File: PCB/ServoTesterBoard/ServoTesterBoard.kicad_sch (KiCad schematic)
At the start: 23 parts, among them J1 Barrel Jack, J2 2.54mm 1x2 Header, J3 2.54mm 1x3 Header, Q1 BC547, SW1 Slide Switch, SW2 Push Button, SW3 Push Button, U1 LM555xM, U2 L7805

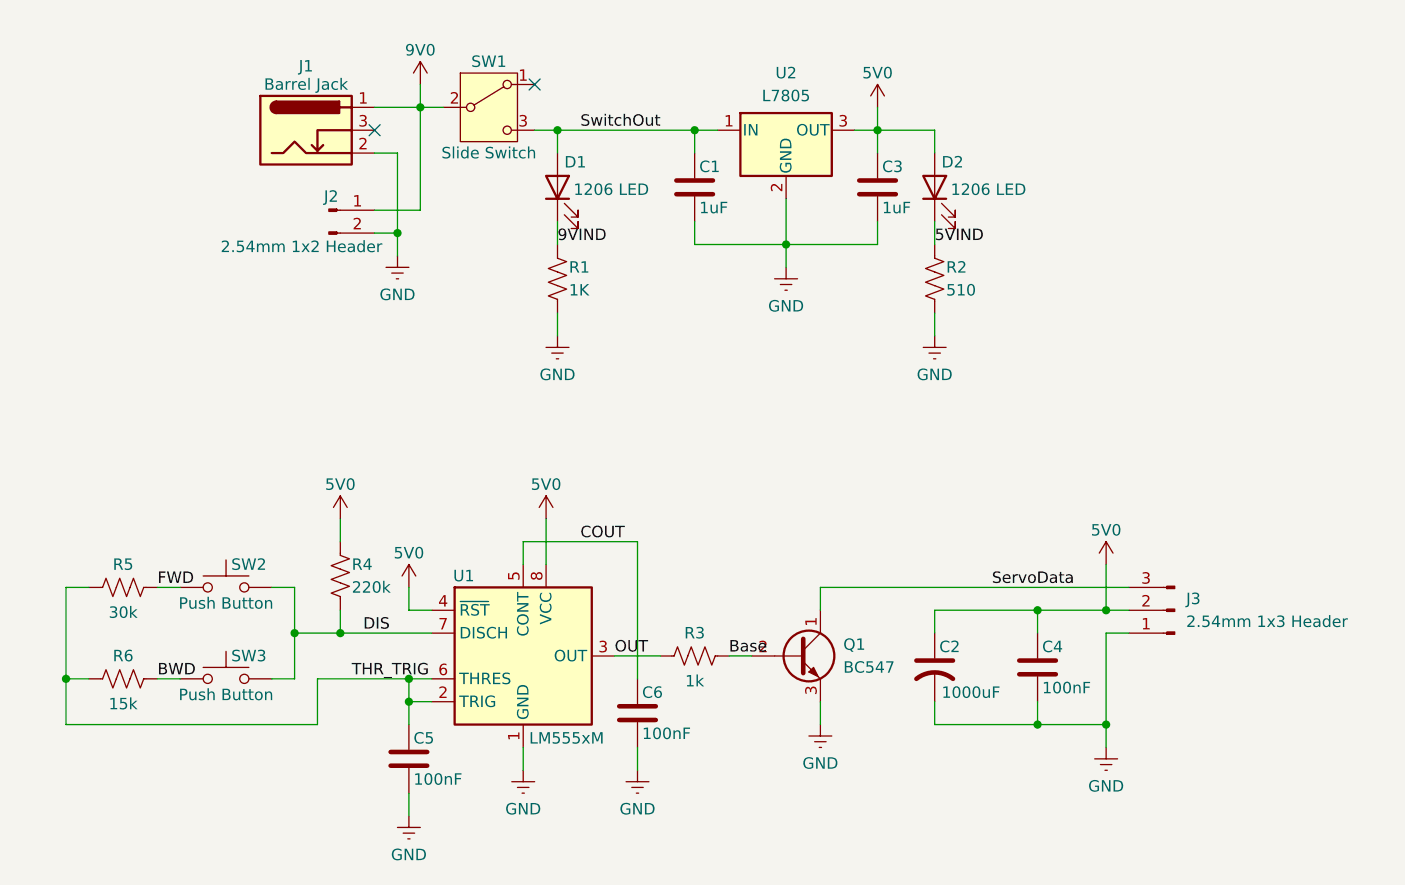
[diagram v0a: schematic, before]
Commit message: Finished
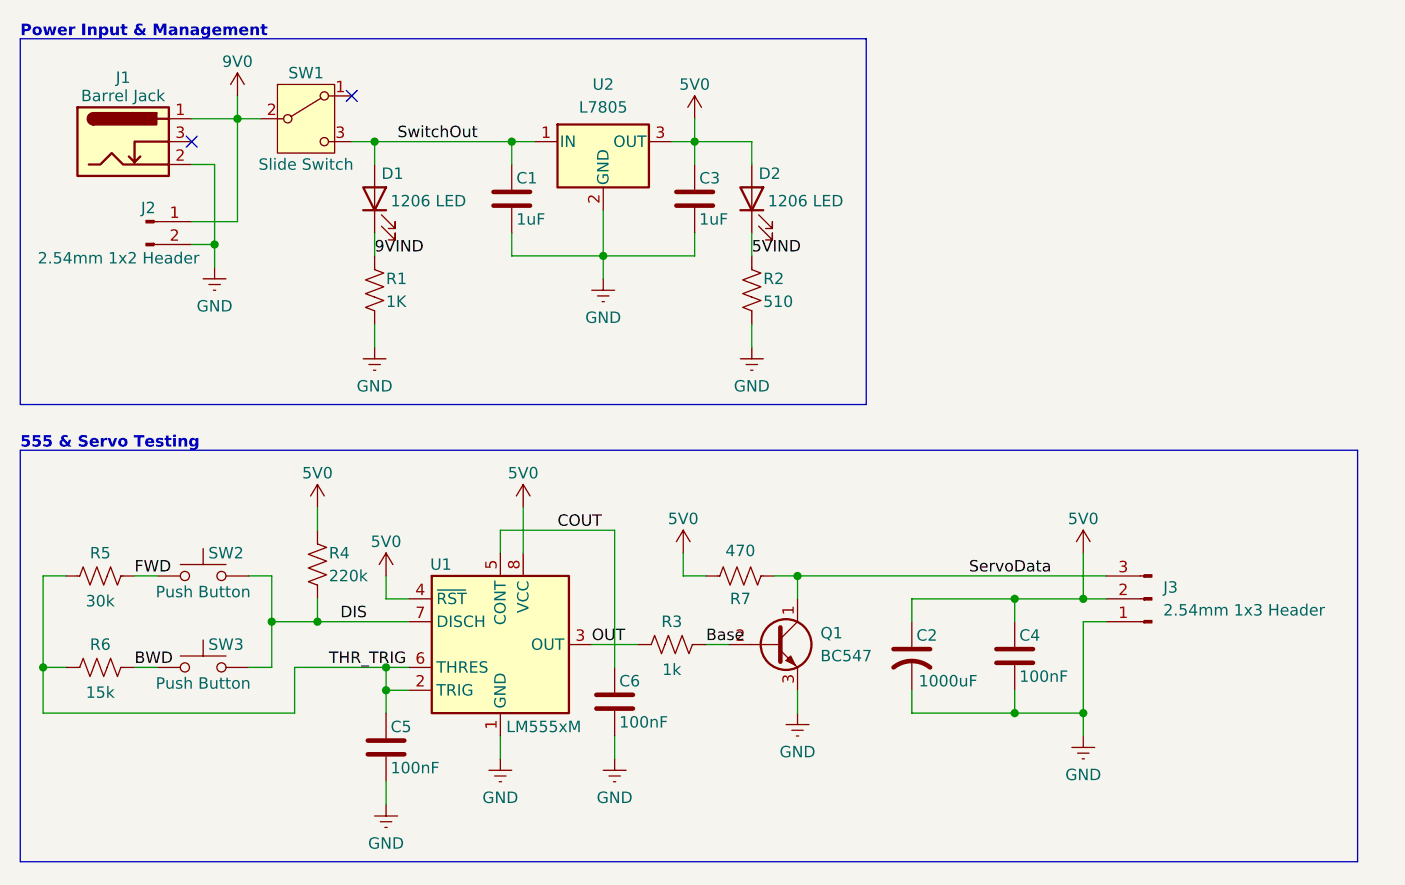
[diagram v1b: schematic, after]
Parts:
- added R7: 470, Resistor_SMD:R_1206_3216Metric_Pad1.30x1.75mm_HandSolder, symbol Device:R_US
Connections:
- net 5V0: now also R7.2
- net ServoData: now also R7.1
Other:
- note added: "555 & Servo Testing"
- note added: "Power Input & Management"
- company: (none) -> Nicholas Niles
- title: (none) -> Servo Tester
- moved on the sheet: C1, C2, C3, C4, C5, C6, D1, D2, J1, J2, J3, Q1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
